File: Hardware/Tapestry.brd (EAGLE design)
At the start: 100 x 80 mm, 81 parts, among them U1 ATSAMS70NXXA-AN, U2 AK4618VQ, U3 V_REG_MIC2920, U4 V_REG_MIC2920, U5 USD-SOCKETNEW, Y1 12MHZ

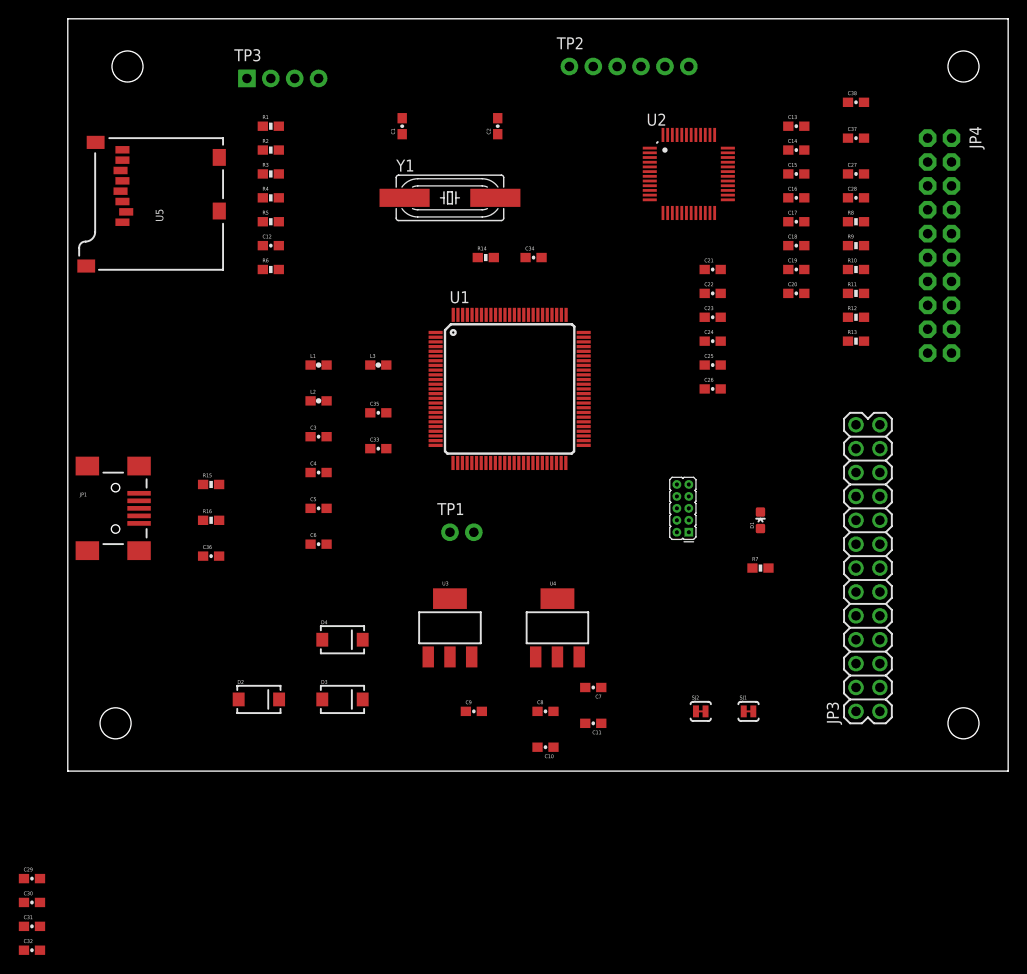
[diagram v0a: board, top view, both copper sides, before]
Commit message: Second update from Jamie
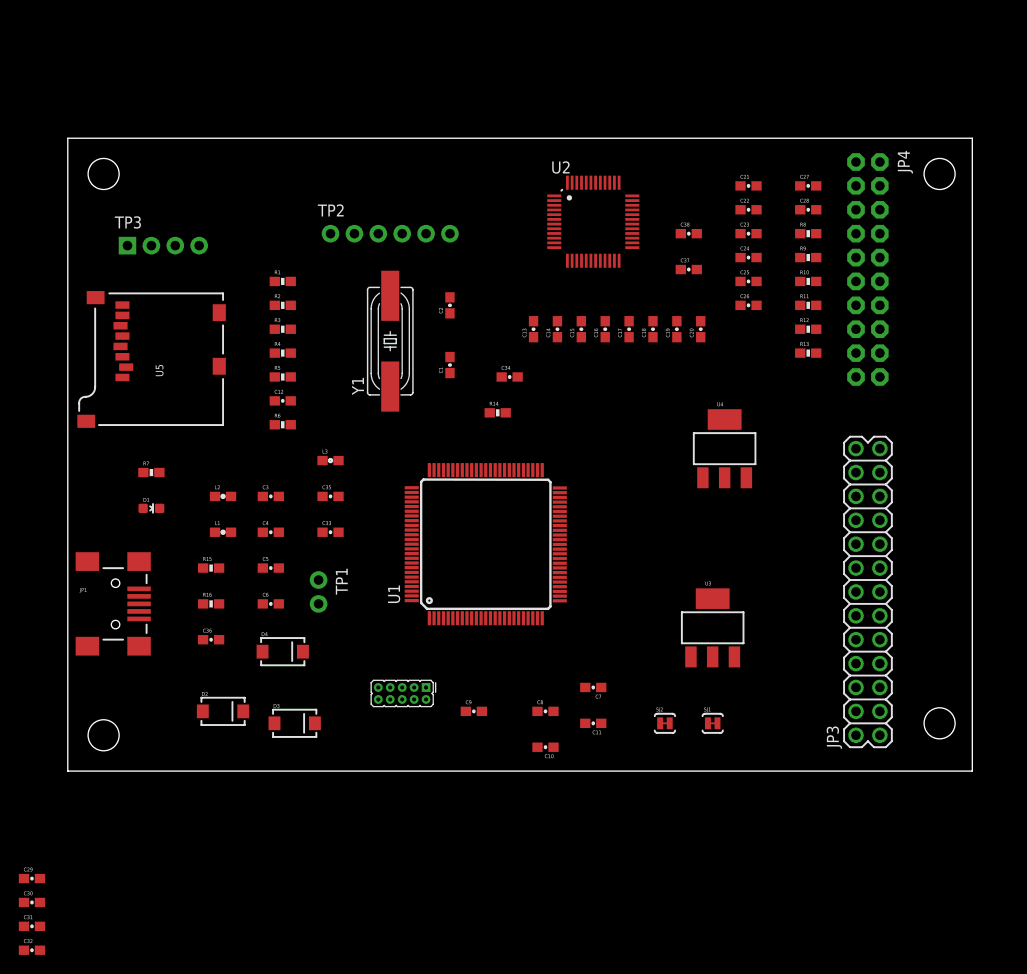
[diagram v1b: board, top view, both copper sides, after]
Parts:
- R15: value 330 -> 15K
- R16: value 330 -> 22K
- moved R7 65.6 mm to (8.89, 31.8)
- moved D1 64.8 mm to (8.89, 27.9), turned to 270 degrees
- moved JP2 41.2 mm to (31.8, 8.89), turned to 270 degrees
- moved C13 35.3 mm to (49.5, 47.0), turned to 90 degrees
- moved C14 31.8 mm to (52.1, 47.0), turned to 90 degrees
- moved TP2 31.0 mm to (27.9, 57.1)
- moved C15 28.2 mm to (54.6, 47.0), turned to 90 degrees
- moved U3 27.9 mm to (68.6, 15.2)
- moved U4 26.1 mm to (69.8, 34.3)
- moved C1 25.9 mm to (40.6, 43.2)
- moved C16 24.7 mm to (57.1, 47.0), turned to 90 degrees
- moved C38 22.6 mm to (66.0, 57.1)
- moved C37 22.6 mm to (66.0, 53.3)
- moved TP3 21.8 mm to (6.35, 55.9)
- moved C17 21.1 mm to (59.7, 47.0), turned to 90 degrees
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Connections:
- removed net RD: TP2.6
- removed net TD: TP2.5
- net TDMI: now also TP2.6
- net TDMO: now also TP2.5
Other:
- board size 100 x 80 mm -> 96.2 x 67.3 mm
